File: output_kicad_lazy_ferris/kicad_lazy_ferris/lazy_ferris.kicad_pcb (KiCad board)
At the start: 2 copper layers, 113.5 x 86.8 mm, 38 parts

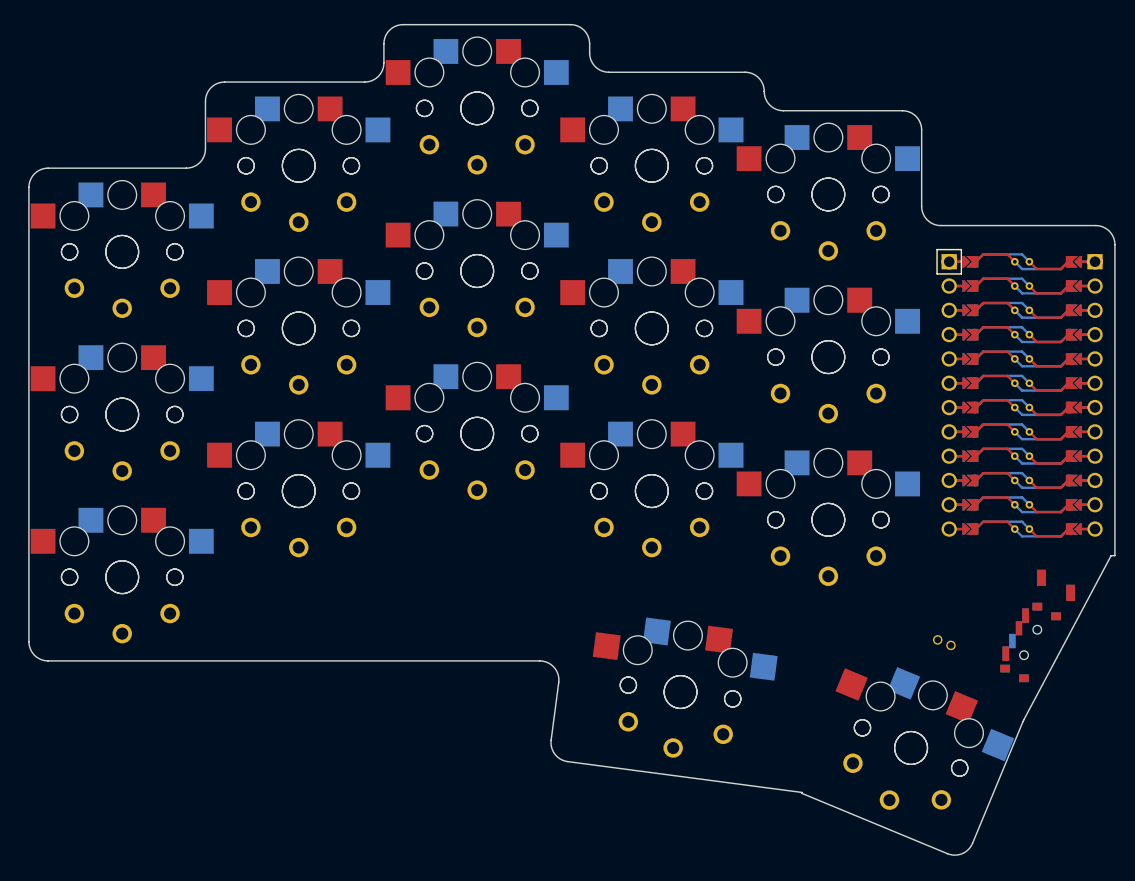
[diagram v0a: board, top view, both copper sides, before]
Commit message: final commit of ergogen v3
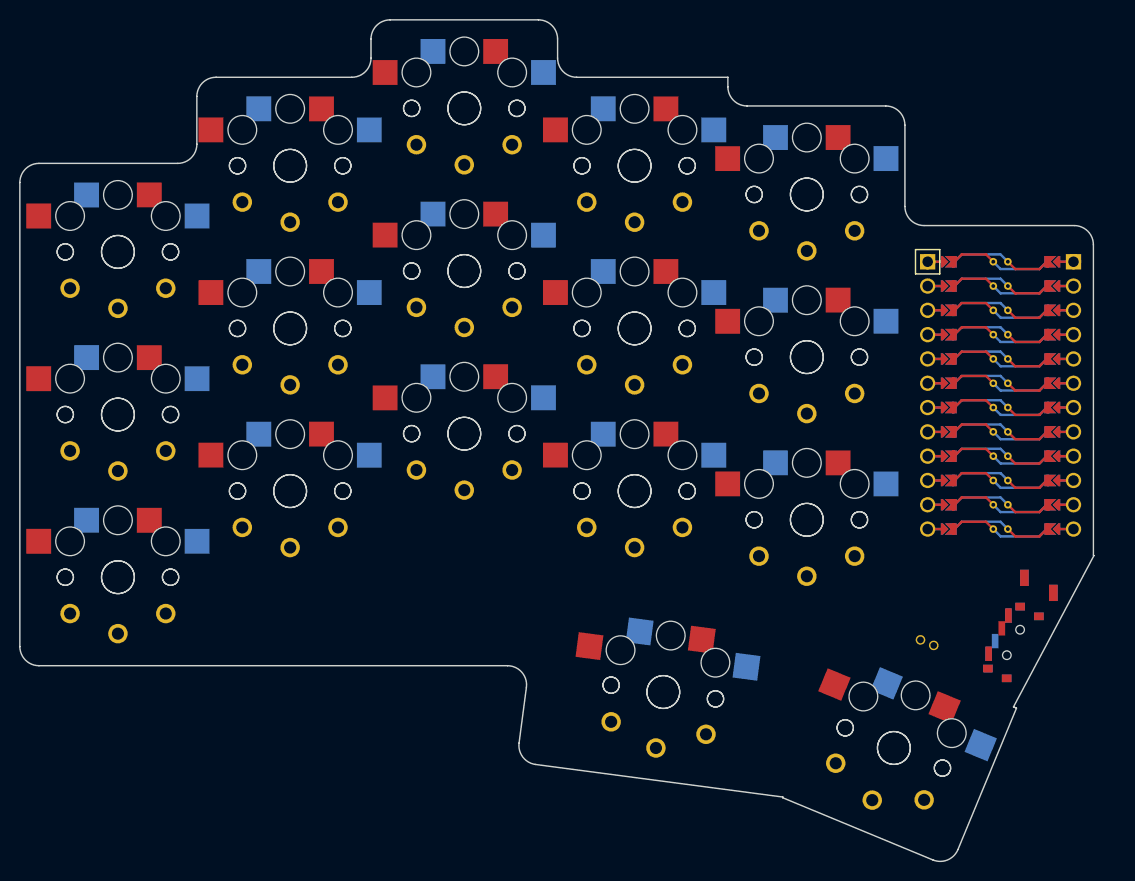
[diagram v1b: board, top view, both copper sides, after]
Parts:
- moved MCU1 2.25 mm to (110.2, -19.0)
- moved S25 2.25 mm to (90.0, -6.00)
- moved S26 2.25 mm to (90.0, -6.00)
- moved S27 2.25 mm to (90.0, -23.0)
- moved S28 2.25 mm to (90.0, -23.0)
- moved S29 2.25 mm to (90.0, -40.0)
- moved S30 2.25 mm to (90.0, -40.0)
- moved ? 1.80 mm to (111.3, 6.67)
- moved ? 1.80 mm to (114.3, 0.85)
- moved ? 1.80 mm to (102.6, 6.84)
- moved S19 1.80 mm to (72.0, -9.00)
- moved S20 1.80 mm to (72.0, -9.00)
- moved S21 1.80 mm to (72.0, -26.0)
- moved S22 1.80 mm to (72.0, -26.0)
- moved S23 1.80 mm to (72.0, -43.0)
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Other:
- board size 113.5 x 86.8 mm -> 112.3 x 88 mm
